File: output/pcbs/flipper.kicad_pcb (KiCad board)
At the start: 2 copper layers, 148.5 x 108.8 mm, 58 parts

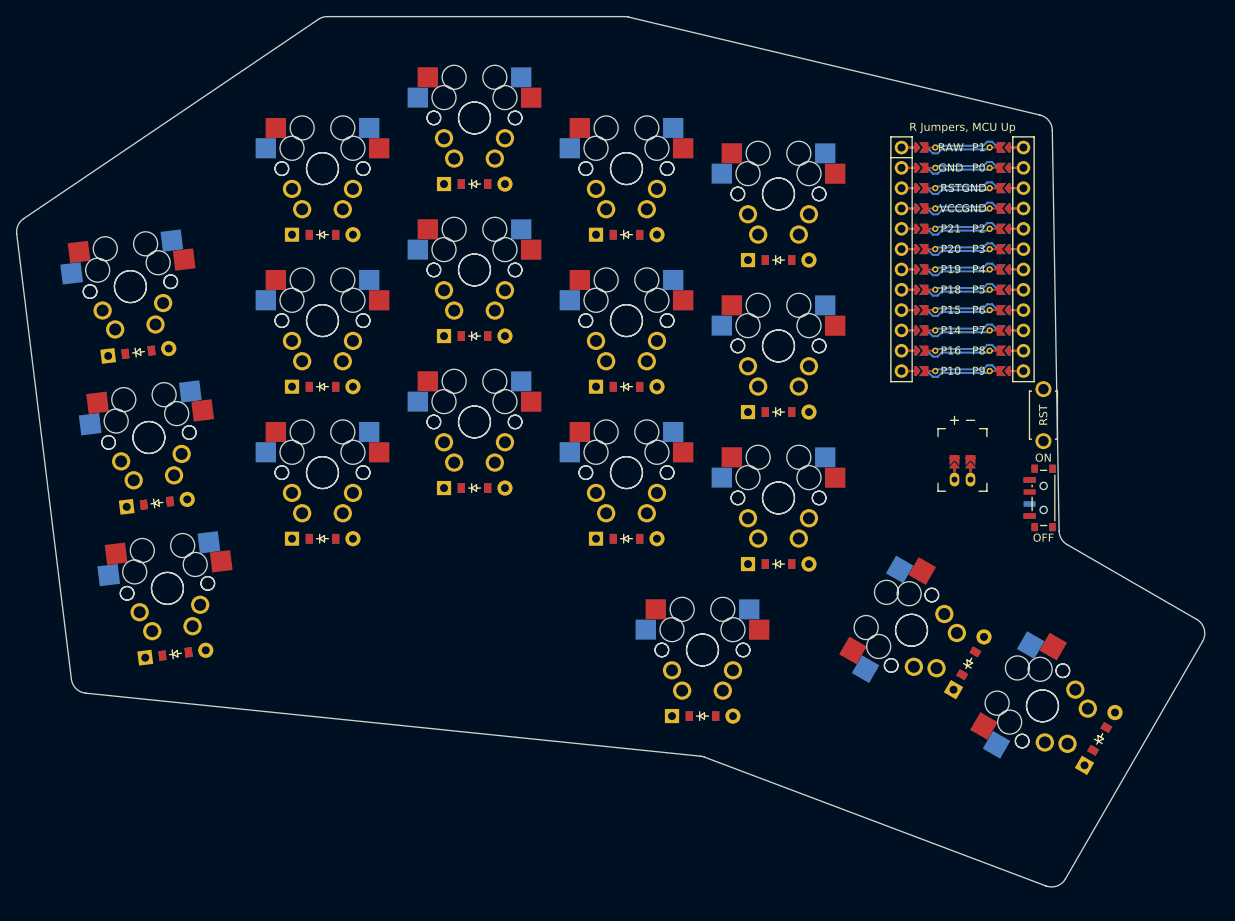
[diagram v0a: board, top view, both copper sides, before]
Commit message: resize
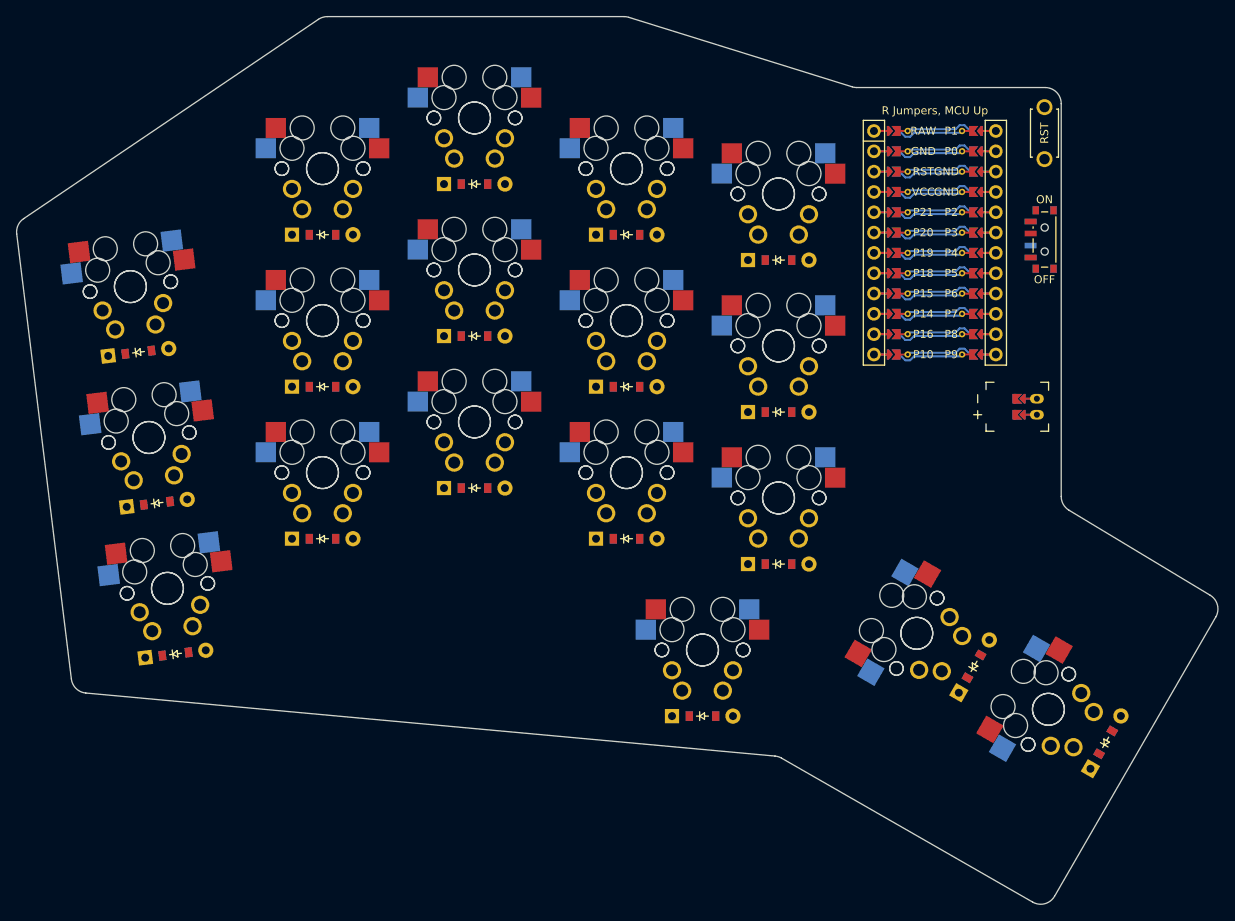
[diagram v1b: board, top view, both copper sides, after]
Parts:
- moved RST1 35.3 mm to (219.1, 30.4)
- moved PWR1 32.3 mm to (219.1, 43.7)
- moved JST1 13.0 mm to (218.1, 64.6), turned to -90 degrees
- moved MCU1 4.02 mm to (205.4, 42.8)
- moved D18 0.86 mm to (226.7, 106.6)
- moved S18 0.86 mm to (219.6, 102.4)
- moved S36 0.86 mm to (219.6, 102.4)
- moved S17 0.76 mm to (203.1, 92.9)
- moved S35 0.76 mm to (203.1, 92.9)
- moved D17 0.76 mm to (210.3, 97.1)
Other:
- board size 148.5 x 108.8 mm -> 150.2 x 111 mm
